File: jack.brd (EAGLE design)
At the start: 44.2 x 26.4 mm, 35 parts, among them IC1 NUF2221W1T2G, IC2 ATSAMD21G18, IC3 LDO, J1 USB-micro, SW1 SPST3.5X6MM, X1 CX-3225 12.288MHz

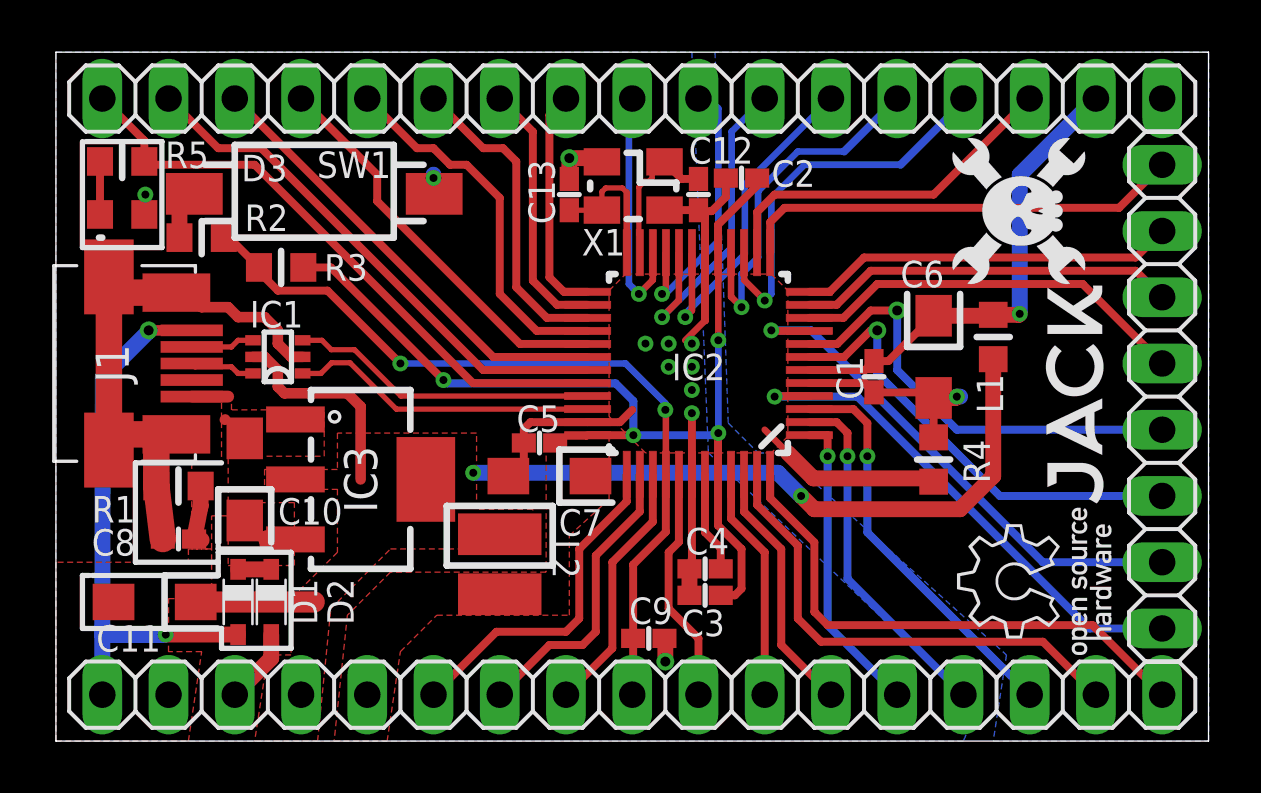
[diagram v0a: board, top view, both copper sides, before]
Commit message: Minor changes (added BOM)
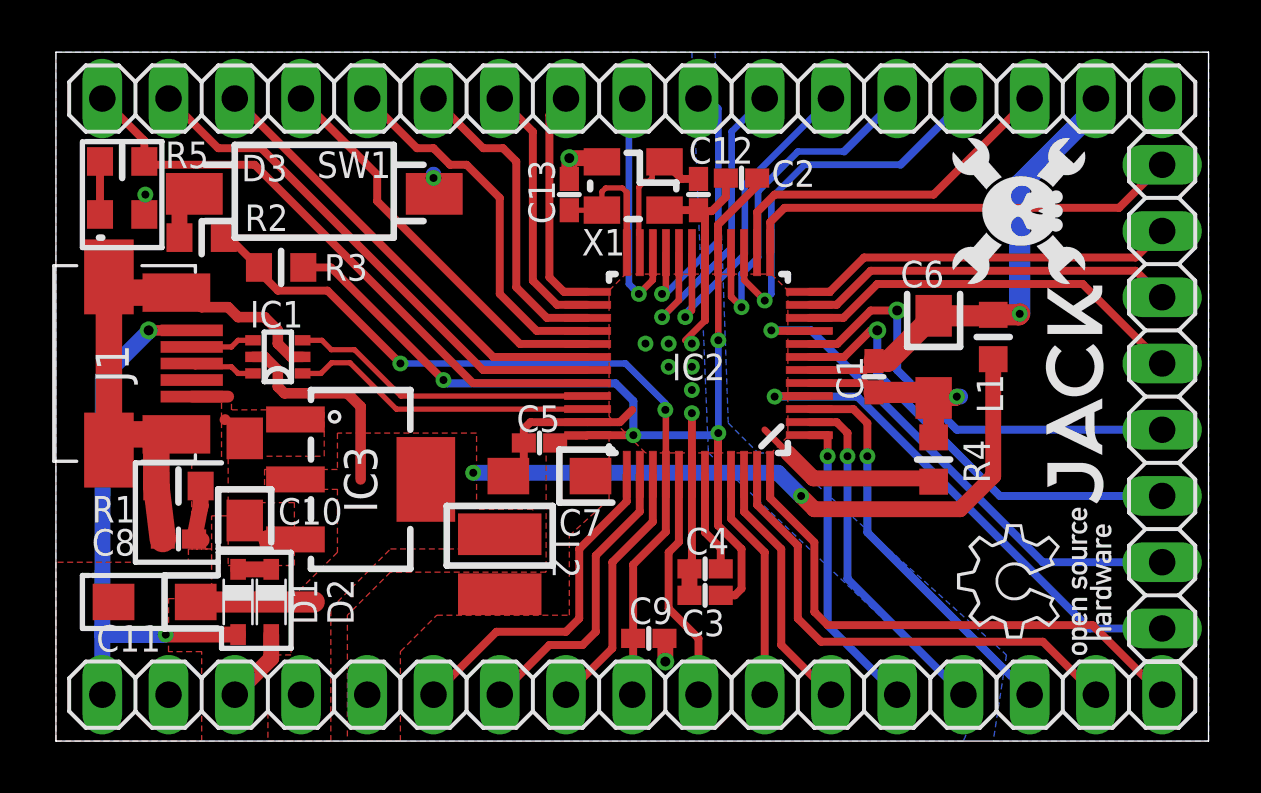
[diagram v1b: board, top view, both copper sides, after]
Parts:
- C10: value 100nF -> 10uF
- C4: device rcl:C0402K -> jack:C0402K
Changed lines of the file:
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@@
 <layer number="45" name="Holes" color="7" fill="1" visible="no" active="yes"/>
 <layer number="46" name="Milling" color="3" fill="1" visible="no" active="yes"/>
-<layer number="47" name="Measures" color="7" fill="1" visible="no" active="yes"/>
+<layer number="47" name="Measures" color="7" fill="1" visible="yes" active="yes"/>
 <layer number="48" name="Document" color="7" fill="1" visible="no" active="yes"/>
 <layer number="49" name="Reference" color="7" fill="1" visible="no" active="yes"/>
 <layer number="50" name="dxf" color="7" fill="1" visible="no" active="no"/>
-<layer number="51" name="tDocu" color="15" fill="1" visible="no" active="yes"/>
+<layer number="51" name="tDocu" color="15" fill="1" visible="yes" active="yes"/>
 <layer number="52" name="bDocu" color="7" fill="1" visible="no" active="yes"/>
 <layer number="53" name="tGND_GNDA" color="7" fill="1" visible="no" active="no"/>
@@
 <attribute name="VALUE" x="29.919" y="14.47" size="1.016" layer="27" rot="R270"/>
 </element>
-<element name="C10" library="jack" package="SMC_P" value="100nF" x="7.239" y="10.033" smashed="yes" rot="R90">
+<element name="C10" library="jack" package="SMC_P" value="10uF" x="7.239" y="10.033" smashed="yes" rot="R90">
 <attribute name="NAME" x="8.517" y="8.299" size="1.016" layer="25"/>
 <attribute name="VALUE" x="8.689" y="9.533" size="1.016" layer="27" rot="R90"/>
@@
 <attribute name="VALUE" x="25.392" y="7.038" size="1.016" layer="27" rot="R180"/>
 </element>
-<element name="C4" library="rcl" package="C0402K" value="100nF" x="24.892" y="6.604" smashed="yes" rot="R180">
+<element name="C4" library="jack" package="C0402K" value="100nF" x="24.892" y="6.604" smashed="yes" rot="R180">
 <attribute name="NAME" x="24.138" y="7.156" size="1.016" layer="25"/>
 <attribute name="VALUE" x="25.392" y="8.054" size="1.016" layer="27" rot="R180"/>
@@
 <vertex x="0" y="6.858"/>
 <vertex x="0" y="0"/>
-<vertex x="5.08" y="0"/>
+<vertex x="5.588" y="0"/>
 <vertex x="5.588" y="3.429"/>
 <vertex x="4.318" y="3.429"/>
@@
 <vertex x="9.017" y="3.302"/>
 <vertex x="8.128" y="3.302"/>
-<vertex x="7.62" y="0"/>
-<vertex x="10.033" y="0"/>
+<vertex x="8.128" y="0"/>
+<vertex x="10.541" y="0"/>
 <vertex x="10.541" y="5.08"/>
 <vertex x="12.827" y="7.366"/>
@@
 <contactref element="L1" pad="2"/>
 <wire x1="28.888" y1="14.228" x2="31.027" y2="14.228" width="0.3048" layer="1"/>
-<wire x1="31.369" y1="14.57" x2="31.918" y2="14.57" width="0.3048" layer="1"/>
-<wire x1="31.918" y1="14.57" x2="33.655" y2="16.307" width="0.3048" layer="1"/>
 <wire x1="31.027" y1="14.228" x2="31.369" y2="14.57" width="0.3048" layer="1"/>
-<wire x1="33.655" y1="16.307" x2="35.904" y2="16.307" width="0.6096" layer="1"/>
-<wire x1="35.904" y1="16.307" x2="35.941" y2="16.344" width="0.6096" layer="1"/>
 <contactref element="JP2" pad="16"/>
-<wire x1="35.941" y1="16.344" x2="36.918" y2="16.344" width="0.6096" layer="1"/>
-<wire x1="36.918" y1="16.344" x2="36.957" y2="16.383" width="0.6096" layer="1"/>
 <via x="36.957" y="16.383" extent="1-16" drill="0.3048" diameter="0.6096"/>
-<wire x1="36.957" y1="16.383" x2="36.957" y2="21.717" width="0.6096" layer="16"/>
-<wire x1="36.957" y1="21.717" x2="39.878" y2="24.638" width="0.6096" layer="16"/>
+<wire x1="31.369" y1="14.57" x2="31.918" y2="14.57" width="0.8128" layer="1"/>
+<wire x1="31.918" y1="14.57" x2="33.655" y2="16.307" width="0.8128" layer="1"/>
+<wire x1="33.655" y1="16.307" x2="35.904" y2="16.307" width="0.8128" layer="1"/>
+<wire x1="35.904" y1="16.307" x2="35.941" y2="16.344" width="0.8128" layer="1"/>
+<wire x1="35.941" y1="16.344" x2="36.918" y2="16.344" width="0.8128" layer="1"/>
+<wire x1="36.918" y1="16.344" x2="36.957" y2="16.383" width="0.8128" layer="1"/>
+<wire x1="36.957" y1="16.383" x2="36.957" y2="21.336" width="0.8128" layer="16"/>
+<wire x1="36.957" y1="21.336" x2="39.624" y2="24.003" width="0.8128" layer="16"/>
+<wire x1="39.624" y1="24.003" x2="39.624" y2="24.384" width="0.8128" layer="16"/>
+<wire x1="39.624" y1="24.384" x2="39.878" y2="24.638" width="0.8128" layer="16"/>
 </signal>
 <signal name="D+OUT">
@@
 <vertex x="12.827" y="6.477"/>
 <vertex x="11.176" y="4.826"/>
-<vertex x="10.668" y="0"/>
-<vertex x="12.7" y="0"/>
+<vertex x="11.176" y="0"/>
+<vertex x="13.208" y="0"/>
 <vertex x="13.208" y="3.429"/>
 <vertex x="14.605" y="4.826"/>
@@
 </polygon>
 <wire x1="33.442" y1="13.37" x2="33.655" y2="13.157" width="0.3048" layer="1"/>
-<wire x1="33.655" y1="11.645" x2="33.655" y2="13.157" width="0.3048" layer="1"/>
-<wire x1="31.369" y1="13.37" x2="33.442" y2="13.37" width="0.3048" layer="1"/>
 <wire x1="31.011" y1="13.728" x2="31.369" y2="13.37" width="0.3048" layer="1"/>
 <wire x1="33.655" y1="13.157" x2="34.493" y2="13.157" width="0.6096" layer="1"/>
@@
 <wire x1="34.544" y1="13.208" x2="34.671" y2="13.208" width="0.6096" layer="16"/>
 <contactref element="JP2" pad="17"/>
+<wire x1="33.655" y1="11.645" x2="33.655" y2="13.157" width="0.8128" layer="1"/>
+<wire x1="31.369" y1="13.37" x2="33.655" y2="13.37" width="0.8128" layer="1"/>
+<wire x1="33.655" y1="13.37" x2="33.655" y2="13.157" width="0.8128" layer="1"/>
 </signal>
 <signal name="SWCLK">
